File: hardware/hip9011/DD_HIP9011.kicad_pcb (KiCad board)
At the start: 2 copper layers, 40 x 34 mm, 37 parts, among them P161 KNOCK 1, P162 KNOCK 2, P163 12V, P164 CONN_5X2, P165 CONN_2, P166 CONN_2, U131 7805-SOT89, X161 CRYSTAL

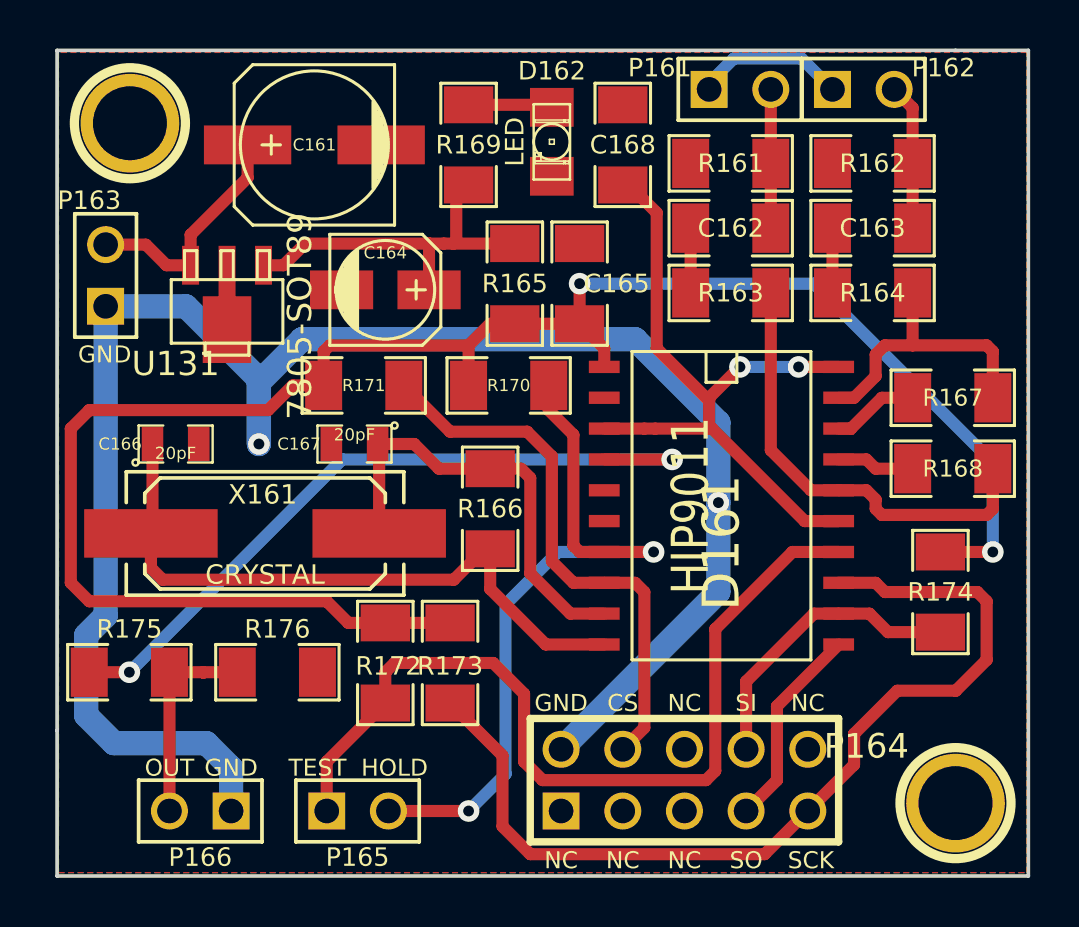
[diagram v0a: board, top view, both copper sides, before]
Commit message: update pcb files
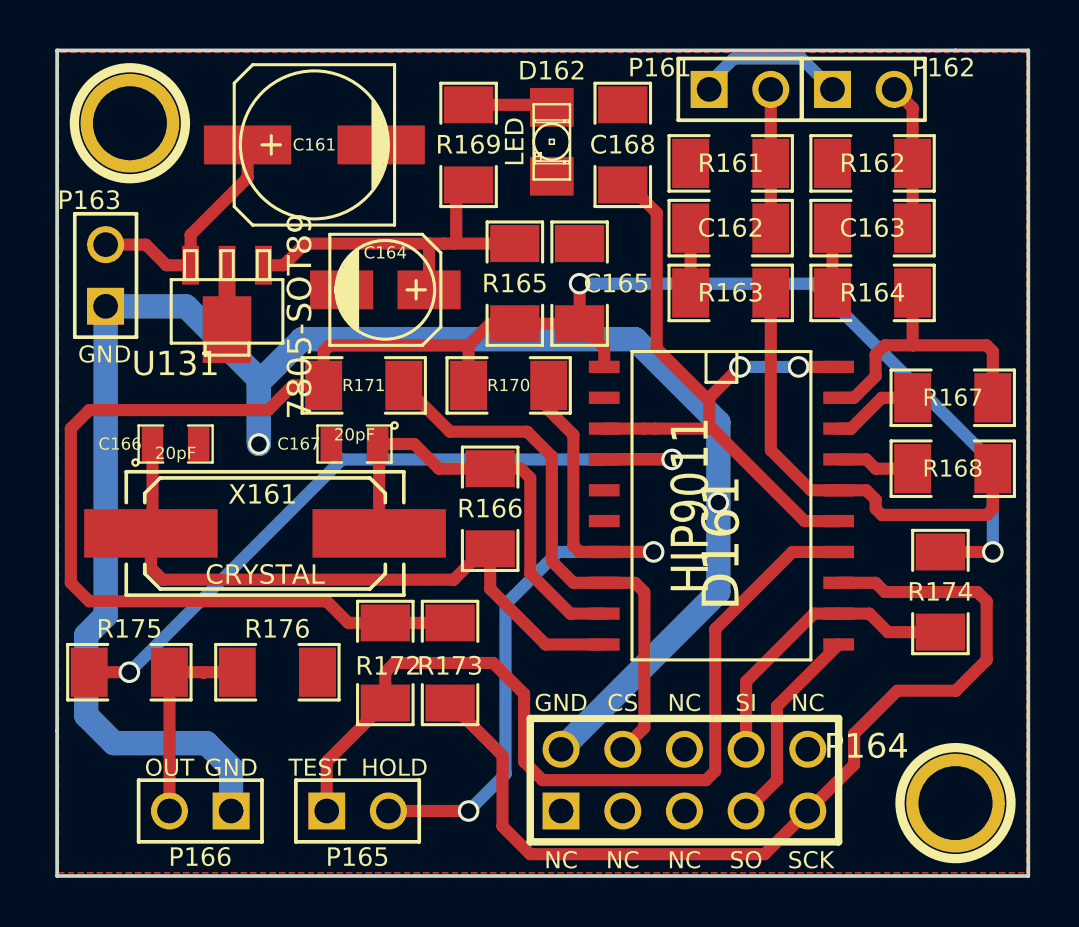
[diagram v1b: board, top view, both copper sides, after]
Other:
- net class Default removed
